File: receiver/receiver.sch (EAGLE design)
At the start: 9 parts, among them P1 PROMICRO_HEADER, P2 PROMICRO_HEADER, U1 CORE51822B, U2 3.3

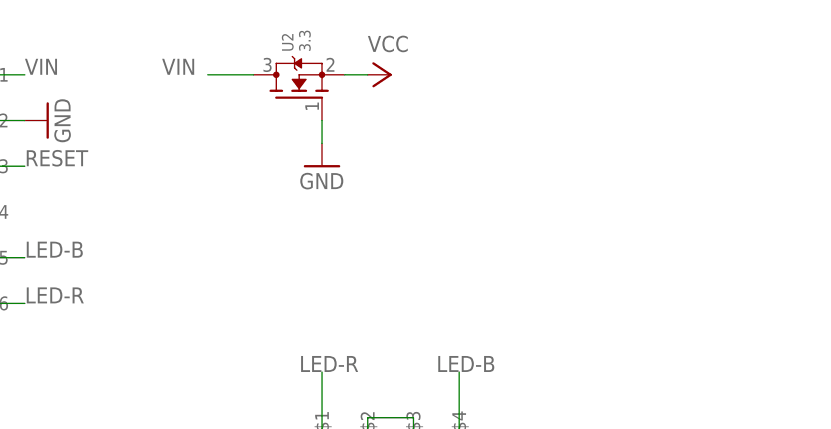
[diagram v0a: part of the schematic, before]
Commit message: update board
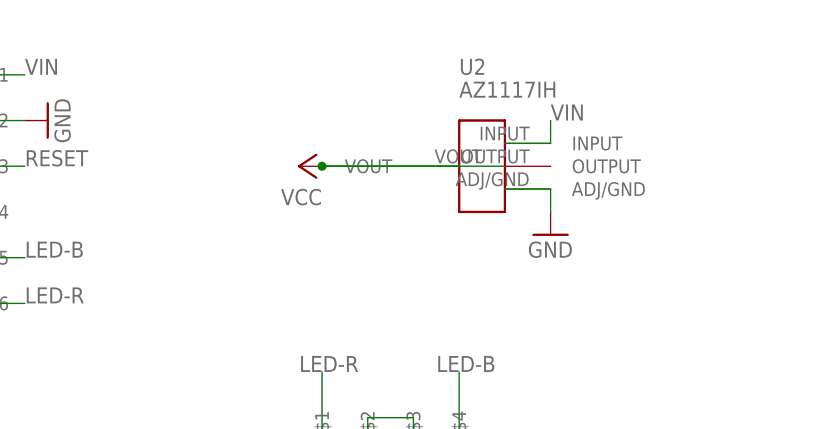
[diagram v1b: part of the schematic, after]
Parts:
- U2: value 3.3 -> AZ1117IH; device adafruit:MOSFET-NREFLOW -> az1117ih:AZ1117IH
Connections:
- net GND: now also U2.ADJ/GND; no longer U2.G
- net VCC: now also U2.OUTPUT, U2.VOUT; no longer U2.S
- net VIN: now also U2.INPUT; no longer U2.D
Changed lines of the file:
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@@
 </classes>
 <parts>
-<part name="U2" library="adafruit" deviceset="MOSFET-N" device="REFLOW" value="3.3"/>
 <part name="GND1" library="supply1" library_urn="urn:adsk.eagle:library:371" deviceset="GND" device=""/>
 <part name="GND2" library="supply1" library_urn="urn:adsk.eagle:library:371" deviceset="GND" device=""/>
@@
 <part name="P2" library="promicro_header" deviceset="PROMICRO_HEADER" device=""/>
 <part name="P1" library="promicro_header" deviceset="PROMICRO_HEADER" device=""/>
+<part name="U2" library="az1117ih" deviceset="AZ1117IH" device=""/>
 </parts>
 <sheets>
@@
 </plain>
 <instances>
-<instance part="U2" gate="G$1" x="96.52" y="119.38" rot="R90"/>
-<instance part="GND1" gate="1" x="99.06" y="111.76"/>
+<instance part="GND1" gate="1" x="124.46" y="104.14"/>
 <instance part="GND2" gate="1" x="68.58" y="116.84" rot="R90"/>
 <instance part="GND3" gate="1" x="-20.32" y="76.2"/>
 <instance part="GND4" gate="1" x="30.48" y="109.22" rot="R90"/>
-<instance part="P+1" gate="VCC" x="106.68" y="121.92" rot="R270"/>
+<instance part="P+1" gate="VCC" x="96.52" y="111.76" rot="R90"/>
 <instance part="D1" gate="G$1" x="119.38" y="27.94"/>
 <instance part="RA2" gate="G$1" x="71.12" y="-2.54"/>
@@
 <instance part="P2" gate="G$1" x="53.34" y="109.22"/>
 <instance part="P1" gate="G$1" x="10.16" y="109.22"/>
+<instance part="U2" gate="G$1" x="116.84" y="111.76"/>
 </instances>
 <busses>
@@
 <nets>
 <net name="GND" class="0">
-<segment>
-<pinref part="GND1" gate="1" pin="GND"/>
-<pinref part="U2" gate="G$1" pin="G"/>
-<wire x1="99.06" y1="114.3" x2="99.06" y2="116.84" width="0.1524" layer="91"/>
-</segment>
 <segment>
 <pinref part="GND2" gate="1" pin="GND"/>
@@
 <junction x="22.86" y="109.22"/>
 </segment>
+<segment>
+<pinref part="U2" gate="G$1" pin="ADJ/GND"/>
+<pinref part="GND1" gate="1" pin="GND"/>
+<wire x1="124.46" y1="109.22" x2="119.38" y2="109.22" width="0.1524" layer="91"/>
+<wire x1="124.46" y1="109.22" x2="124.46" y2="106.68" width="0.1524" layer="91"/>
+</segment>
 </net>
 <net name="VCC" class="0">
-<segment>
-<pinref part="U2" gate="G$1" pin="S"/>
-<pinref part="P+1" gate="VCC" pin="VCC"/>
-<wire x1="101.6" y1="121.92" x2="104.14" y2="121.92" width="0.1524" layer="91"/>
-</segment>
 <segment>
 <pinref part="U1" gate="G$1" pin="VCC"/>
@@
 <wire x1="10.16" y1="33.02" x2="2.54" y2="33.02" width="0.1524" layer="91"/>
 <wire x1="2.54" y1="33.02" x2="2.54" y2="27.94" width="0.1524" layer="91"/>
+</segment>
+<segment>
+<pinref part="U2" gate="G$1" pin="VOUT"/>
+<pinref part="P+1" gate="VCC" pin="VCC"/>
+<wire x1="114.3" y1="111.76" x2="99.06" y2="111.76" width="0.1524" layer="91"/>
+<pinref part="U2" gate="G$1" pin="OUTPUT"/>
+<wire x1="119.38" y1="111.76" x2="99.06" y2="111.76" width="0.1524" layer="91"/>
+<junction x="99.06" y="111.76"/>
 </segment>
 </net>
@@
 </segment>
 <segment>
-<pinref part="U2" gate="G$1" pin="D"/>
-<wire x1="91.44" y1="121.92" x2="86.36" y2="121.92" width="0.1524" layer="91"/>
-<label x="81.28" y="121.92" size="1.778" layer="95"/>
-</segment>
-<segment>
 <pinref part="D1" gate="G$1" pin="COMM(ANODE)"/>
 <wire x1="111.76" y1="25.4" x2="106.68" y2="25.4" width="0.1524" layer="91"/>
@@
 <label x="104.14" y="15.24" size="1.778" layer="95"/>
 </segment>
-</net>
+<segment>
+<pinref part="U2" gate="G$1" pin="INPUT"/>
+<wire x1="119.38" y1="114.3" x2="124.46" y2="114.3" width="0.1524" layer="91"/>
+<wire x1="124.46" y1="114.3" x2="124.46" y2="116.84" width="0.1524" layer="91"/>
+<label x="124.46" y="116.84" size="1.778" layer="95"/>
+</segment>
+</net>
